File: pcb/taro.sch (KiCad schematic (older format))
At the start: 35 parts, among them J1 Conn_01x04_Female, SW1 Reset, SW10 SW_Push, SW11 SW_Push, SW12 SW_Push, SW13 SW_Push, SW14 Rotary_Encoder_Switch, SW15 SW_Push, SW16 SW_Push, SW17 SW_Push, SW2 SW_Push, SW3 SW_Push, SW4 SW_Push, SW5 SW_Push, SW6 SW_Push, SW7 SW_Push, SW8 SW_Push, SW9 SW_Push, U1 ProMicro

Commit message: pcb ready for art
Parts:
- SW10, SW11, SW12, SW13, SW15, SW16, SW17, SW2, SW3, SW4, SW5, SW6, SW7, SW8, SW9: footprint TheKeebrary:MX_PCB_100H -> TheKeebrary:Hybrid_PCB_100H
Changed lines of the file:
@@
 F 0 "SW2" H 4400 2585 50  0000 C CNN
 F 1 "SW_Push" H 4400 2494 50  0000 C CNN
-F 2 "TheKeebrary:MX_PCB_100H" H 4400 2500 50  0001 C CNN
+F 2 "TheKeebrary:Hybrid_PCB_100H" H 4400 2500 50  0001 C CNN
 F 3 "~" H 4400 2500 50  0001 C CNN
 	1    4400 2300
@@
 F 0 "SW3" H 4400 3235 50  0000 C CNN
 F 1 "SW_Push" H 4400 3144 50  0000 C CNN
-F 2 "TheKeebrary:MX_PCB_100H" H 4400 3150 50  0001 C CNN
+F 2 "TheKeebrary:Hybrid_PCB_100H" H 4400 3150 50  0001 C CNN
 F 3 "~" H 4400 3150 50  0001 C CNN
 	1    4400 2950
@@
 F 0 "SW4" H 4400 3885 50  0000 C CNN
 F 1 "SW_Push" H 4400 3794 50  0000 C CNN
-F 2 "TheKeebrary:MX_PCB_100H" H 4400 3800 50  0001 C CNN
+F 2 "TheKeebrary:Hybrid_PCB_100H" H 4400 3800 50  0001 C CNN
 F 3 "~" H 4400 3800 50  0001 C CNN
 	1    4400 3600
@@
 F 0 "SW5" H 4400 4535 50  0000 C CNN
 F 1 "SW_Push" H 4400 4444 50  0000 C CNN
-F 2 "TheKeebrary:MX_PCB_100H" H 4400 4450 50  0001 C CNN
+F 2 "TheKeebrary:Hybrid_PCB_100H" H 4400 4450 50  0001 C CNN
 F 3 "~" H 4400 4450 50  0001 C CNN
 	1    4400 4250
@@
 F 0 "SW6" H 5050 2585 50  0000 C CNN
 F 1 "SW_Push" H 5050 2494 50  0000 C CNN
-F 2 "TheKeebrary:MX_PCB_100H" H 5050 2500 50  0001 C CNN
+F 2 "TheKeebrary:Hybrid_PCB_100H" H 5050 2500 50  0001 C CNN
 F 3 "~" H 5050 2500 50  0001 C CNN
 	1    5050 2300
@@
 F 0 "SW7" H 5050 3235 50  0000 C CNN
 F 1 "SW_Push" H 5050 3144 50  0000 C CNN
-F 2 "TheKeebrary:MX_PCB_100H" H 5050 3150 50  0001 C CNN
+F 2 "TheKeebrary:Hybrid_PCB_100H" H 5050 3150 50  0001 C CNN
 F 3 "~" H 5050 3150 50  0001 C CNN
 	1    5050 2950
@@
 F 0 "SW8" H 5050 3885 50  0000 C CNN
 F 1 "SW_Push" H 5050 3794 50  0000 C CNN
-F 2 "TheKeebrary:MX_PCB_100H" H 5050 3800 50  0001 C CNN
+F 2 "TheKeebrary:Hybrid_PCB_100H" H 5050 3800 50  0001 C CNN
 F 3 "~" H 5050 3800 50  0001 C CNN
 	1    5050 3600
@@
 F 0 "SW9" H 5050 4535 50  0000 C CNN
 F 1 "SW_Push" H 5050 4444 50  0000 C CNN
-F 2 "TheKeebrary:MX_PCB_100H" H 5050 4450 50  0001 C CNN
+F 2 "TheKeebrary:Hybrid_PCB_100H" H 5050 4450 50  0001 C CNN
 F 3 "~" H 5050 4450 50  0001 C CNN
 	1    5050 4250
@@
 F 0 "SW13" H 5700 4535 50  0000 C CNN
 F 1 "SW_Push" H 5700 4444 50  0000 C CNN
-F 2 "TheKeebrary:MX_PCB_100H" H 5700 4450 50  0001 C CNN
+F 2 "TheKeebrary:Hybrid_PCB_100H" H 5700 4450 50  0001 C CNN
 F 3 "~" H 5700 4450 50  0001 C CNN
 	1    5700 4250
@@
 F 0 "SW12" H 5700 3885 50  0000 C CNN
 F 1 "SW_Push" H 5700 3794 50  0000 C CNN
-F 2 "TheKeebrary:MX_PCB_100H" H 5700 3800 50  0001 C CNN
+F 2 "TheKeebrary:Hybrid_PCB_100H" H 5700 3800 50  0001 C CNN
 F 3 "~" H 5700 3800 50  0001 C CNN
 	1    5700 3600
@@
 F 0 "SW11" H 5700 3235 50  0000 C CNN
 F 1 "SW_Push" H 5700 3144 50  0000 C CNN
-F 2 "TheKeebrary:MX_PCB_100H" H 5700 3150 50  0001 C CNN
+F 2 "TheKeebrary:Hybrid_PCB_100H" H 5700 3150 50  0001 C CNN
 F 3 "~" H 5700 3150 50  0001 C CNN
 	1    5700 2950
@@
 F 0 "SW10" H 5700 2585 50  0000 C CNN
 F 1 "SW_Push" H 5700 2494 50  0000 C CNN
-F 2 "TheKeebrary:MX_PCB_100H" H 5700 2500 50  0001 C CNN
+F 2 "TheKeebrary:Hybrid_PCB_100H" H 5700 2500 50  0001 C CNN
 F 3 "~" H 5700 2500 50  0001 C CNN
 	1    5700 2300
@@
 F 0 "SW17" H 7850 4535 50  0000 C CNN
 F 1 "SW_Push" H 7850 4444 50  0000 C CNN
-F 2 "TheKeebrary:MX_PCB_100H" H 7850 4450 50  0001 C CNN
+F 2 "TheKeebrary:Hybrid_PCB_100H" H 7850 4450 50  0001 C CNN
 F 3 "~" H 7850 4450 50  0001 C CNN
 	1    7850 4250
@@
 F 0 "SW16" H 7200 4535 50  0000 C CNN
 F 1 "SW_Push" H 7200 4444 50  0000 C CNN
-F 2 "TheKeebrary:MX_PCB_100H" H 7200 4450 50  0001 C CNN
+F 2 "TheKeebrary:Hybrid_PCB_100H" H 7200 4450 50  0001 C CNN
 F 3 "~" H 7200 4450 50  0001 C CNN
 	1    7200 4250
@@
 F 0 "SW15" H 6550 4535 50  0000 C CNN
 F 1 "SW_Push" H 6550 4444 50  0000 C CNN
-F 2 "TheKeebrary:MX_PCB_100H" H 6550 4450 50  0001 C CNN
+F 2 "TheKeebrary:Hybrid_PCB_100H" H 6550 4450 50  0001 C CNN
 F 3 "~" H 6550 4450 50  0001 C CNN
 	1    6550 4250

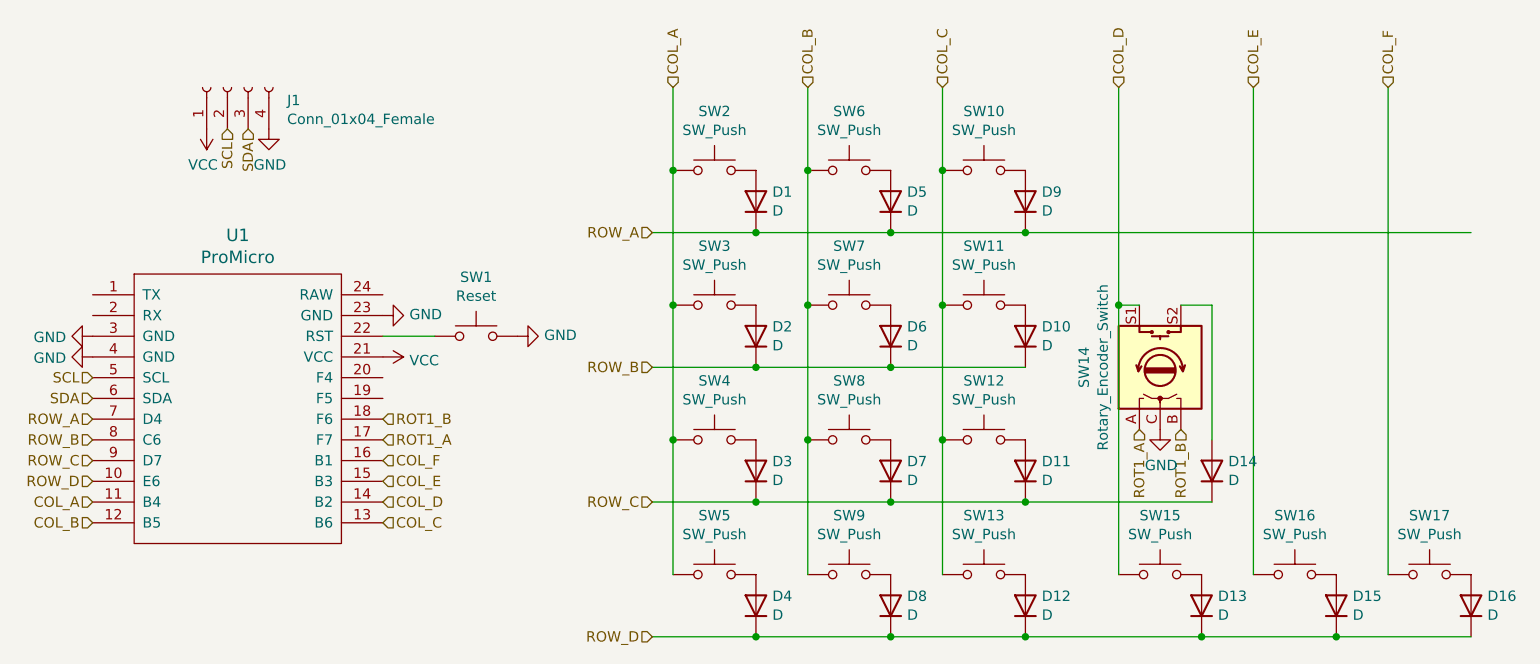
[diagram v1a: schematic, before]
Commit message: pcb done?
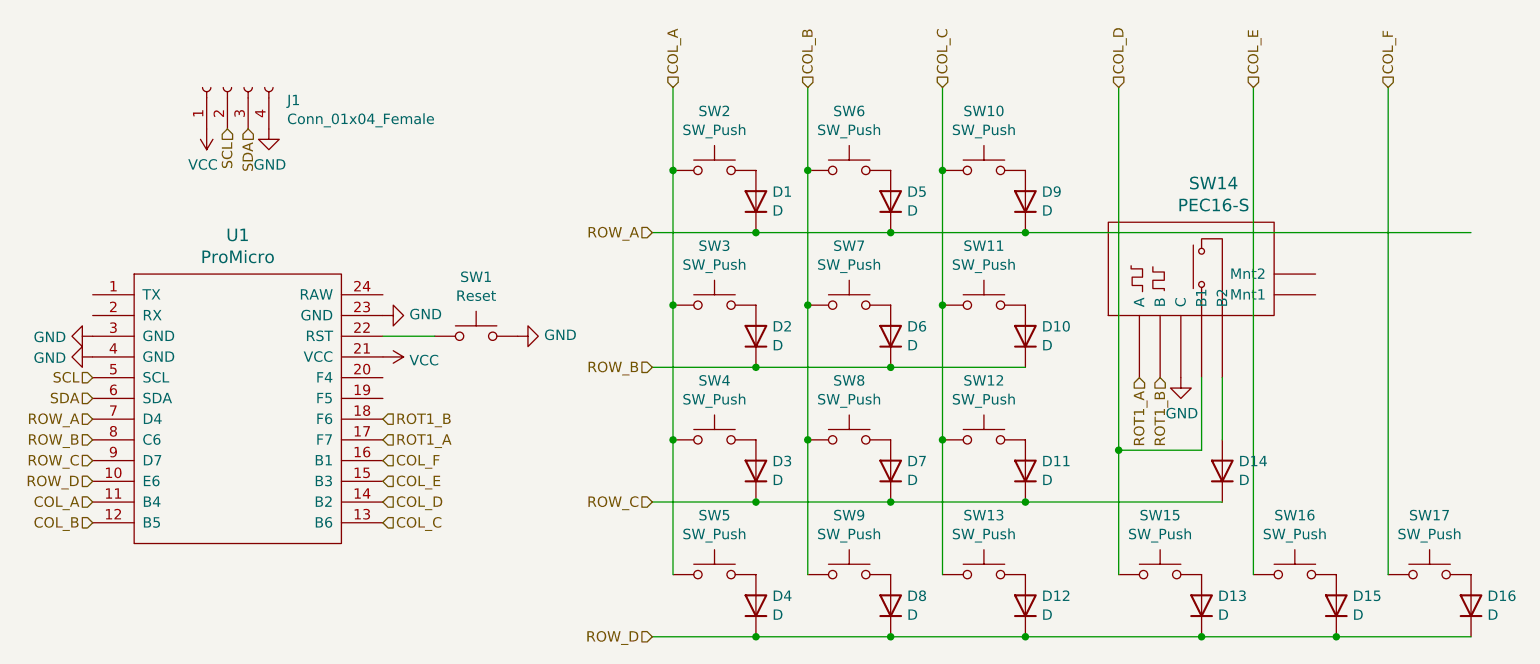
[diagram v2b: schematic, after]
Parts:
- removed SW14: Rotary_Encoder_Switch, Keebio_Parts:RotaryEncoder_Alps_EC11E-Switch_Vertical_H20mm, symbol Device:Rotary_Encoder_Switch
- added SW14: PEC16-S, Avp:PEC16-4xxxF-Sxxxx, symbol avp:PEC16-S
- U1: footprint Keebio_Parts:ArduinoProMicro -> Keebio_Parts:ArduinoProMicro-TopSide
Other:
- moved on the sheet: D14
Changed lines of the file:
@@
 F 0 "U1" H 2100 4687 60  0000 C CNN
 F 1 "ProMicro" H 2100 4581 60  0000 C CNN
-F 2 "Keebio_Parts:ArduinoProMicro" H 2200 2600 60  0001 C CNN
+F 2 "Keebio_Parts:ArduinoProMicro-TopSide" H 2200 2600 60  0001 C CNN
 F 3 "" H 2200 2600 60  0000 C CNN
 	1    2100 3650
@@
 	0    1    1    0
 $EndComp
-$Comp
-L Device:Rotary_Encoder_Switch SW14
-U 1 1 5F5EEC46
-P 6550 3250
-F 0 "SW14" H 6550 3617 50  0000 C CNN
-F 1 "Rotary_Encoder_Switch" H 6550 3526 50  0000 C CNN
-F 2 "Keebio_Parts:RotaryEncoder_Alps_EC11E-Switch_Vertical_H20mm" H 6400 3410 50  0001 C CNN
-F 3 "~" H 6550 3510 50  0001 C CNN
-	1    6550 3250
-	0    -1   -1   0
-$EndComp
 Wire Wire Line
 	5900 4550 6750 4550
 Connection ~ 5900 4550
 Wire Wire Line
-	5900 3900 6800 3900
+	5900 3900 6850 3900
 Connection ~ 5900 3900
 Connection ~ 5900 2600
@@
 L Device:D D14
 U 1 1 5F601314
-P 6800 3750
-F 0 "D14" V 6846 3671 50  0000 R CNN
-F 1 "D" V 6755 3671 50  0000 R CNN
-F 2 "Keebio_Parts:Diode" H 6800 3750 50  0001 C CNN
-F 3 "~" H 6800 3750 50  0001 C CNN
-	1    6800 3750
-	0    -1   -1   0
-$EndComp
-Wire Wire Line
-	6450 2950 6350 2950
-Connection ~ 6350 2950
-Wire Wire Line
-	6350 2950 6350 4250
-Wire Wire Line
-	6650 2950 6800 2950
-Wire Wire Line
-	6800 2950 6800 3600
-Text HLabel 6650 3550 3    50   Input ~ 0
+P 6850 3750
+F 0 "D14" V 6896 3671 50  0000 R CNN
+F 1 "D" V 6805 3671 50  0000 R CNN
+F 2 "Keebio_Parts:Diode" H 6850 3750 50  0001 C CNN
+F 3 "~" H 6850 3750 50  0001 C CNN
+	1    6850 3750
+	0    -1   -1   0
+$EndComp
+Text HLabel 6550 3300 3    50   Input ~ 0
 ROT1_B
-Text HLabel 6450 3550 3    50   Input ~ 0
-ROT1_A
 $Comp
 L power:GND #PWR08
 U 1 1 5F607E28
-P 6550 3550
-F 0 "#PWR08" H 6550 3300 50  0001 C CNN
-F 1 "GND" H 6555 3377 50  0000 C CNN
-F 2 "" H 6550 3550 50  0001 C CNN
-F 3 "" H 6550 3550 50  0001 C CNN
-	1    6550 3550
+P 6650 3300
+F 0 "#PWR08" H 6650 3050 50  0001 C CNN
+F 1 "GND" H 6655 3127 50  0000 C CNN
+F 2 "" H 6650 3300 50  0001 C CNN
+F 3 "" H 6650 3300 50  0001 C CNN
+	1    6650 3300
 	1    0    0    -1
 $EndComp
@@
 SDA
 Wire Wire Line
-	6350 1900 6350 2950
-Wire Wire Line
 	5900 2600 8050 2600
 Wire Wire Line
@@
 Wire Wire Line
 	7000 1900 7000 4250
+$Comp
+L avp:PEC16-S SW14
+U 1 1 5F5DF600
+P 6500 3000
+F 0 "SW14" V 7137 2692 60  0000 C CNN
+F 1 "PEC16-S" V 7031 2692 60  0000 C CNN
+F 2 "Avp:PEC16-4xxxF-Sxxxx" H 6500 3000 60  0001 C CNN
+F 3 "" H 6500 3000 60  0000 C CNN
+	1    6500 3000
+	0    -1   -1   0
+$EndComp
+Wire Wire Line
+	6350 1900 6350 3650
+Wire Wire Line
+	6850 3600 6850 3300
+Text HLabel 6450 3300 3    50   Input ~ 0
+ROT1_A
+Wire Wire Line
+	6750 3300 6750 3650
+Wire Wire Line
+	6750 3650 6350 3650
+Connection ~ 6350 3650
+Wire Wire Line
+	6350 3650 6350 4250
 $EndSCHEMATC
